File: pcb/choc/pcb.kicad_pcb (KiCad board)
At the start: 2 copper layers, 154.2 x 86 mm, 70 parts, among them J1 MJ-4PP-9, J2 USB_C_Receptacle_USB2.0, J3 Conn_01x04_Female, J4 Conn_01x08_Female, SW1 SW_PUSH, SW10 SW_PUSH, SW11 SW_PUSH, SW12 SW_PUSH, SW13 SW_PUSH, SW14 SW_PUSH, SW15 SW_PUSH, SW16 SW_PUSH, SW17 SW_PUSH, SW18 SW_PUSH, SW19 SW_PUSH, SW2 SW_PUSH, SW3 SW_PUSH, SW4 SW_PUSH, SW5 SW_PUSH, SW6 SW_PUSH, SW7 SW_PUSH, SW8 SW_PUSH, SW9 SW_PUSH, U1 rp2040-zero, U2 rp2040-zero, U3 roller

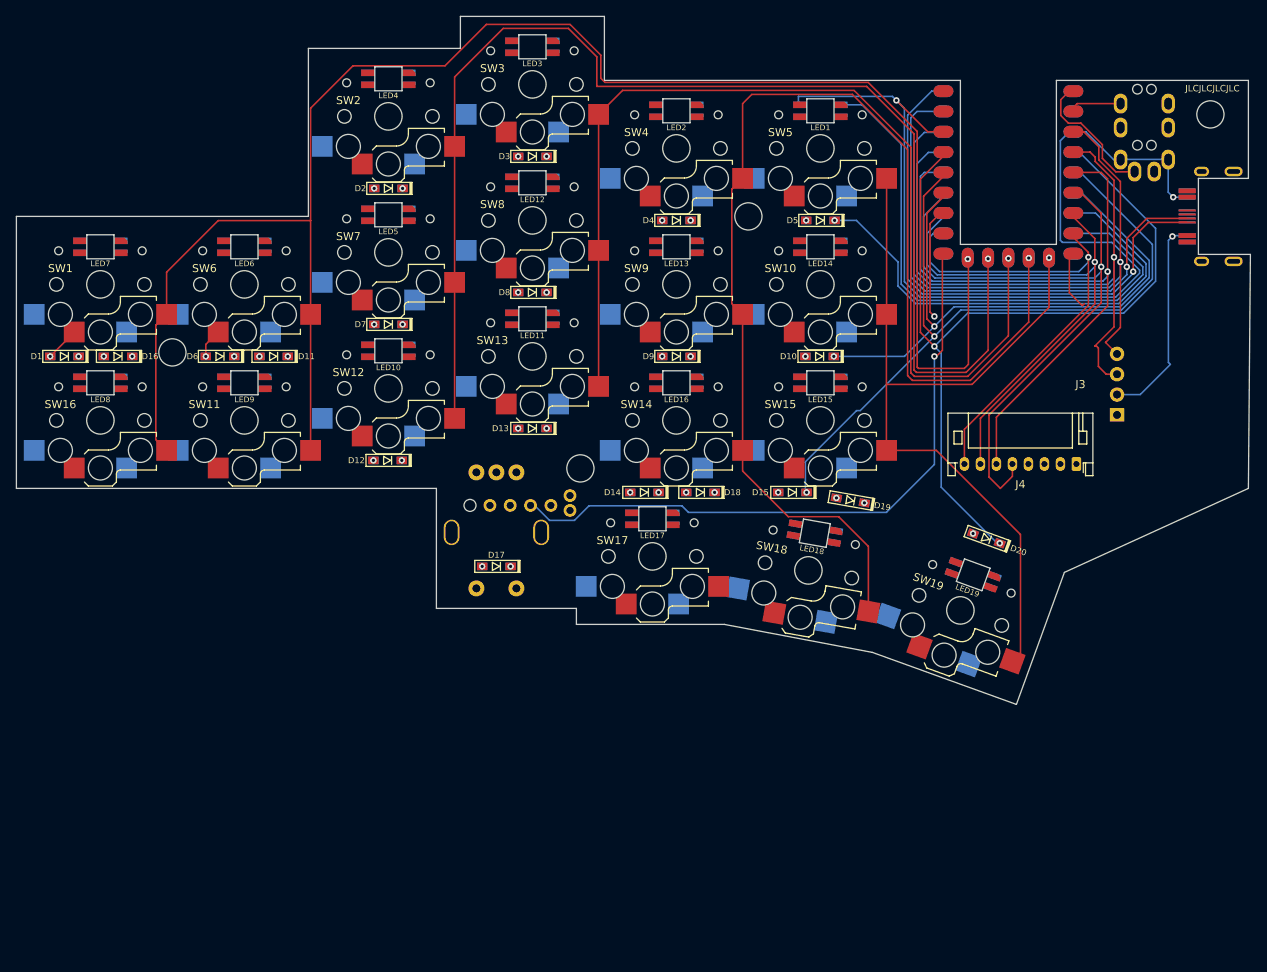
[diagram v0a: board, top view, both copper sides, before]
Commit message: prototype 1
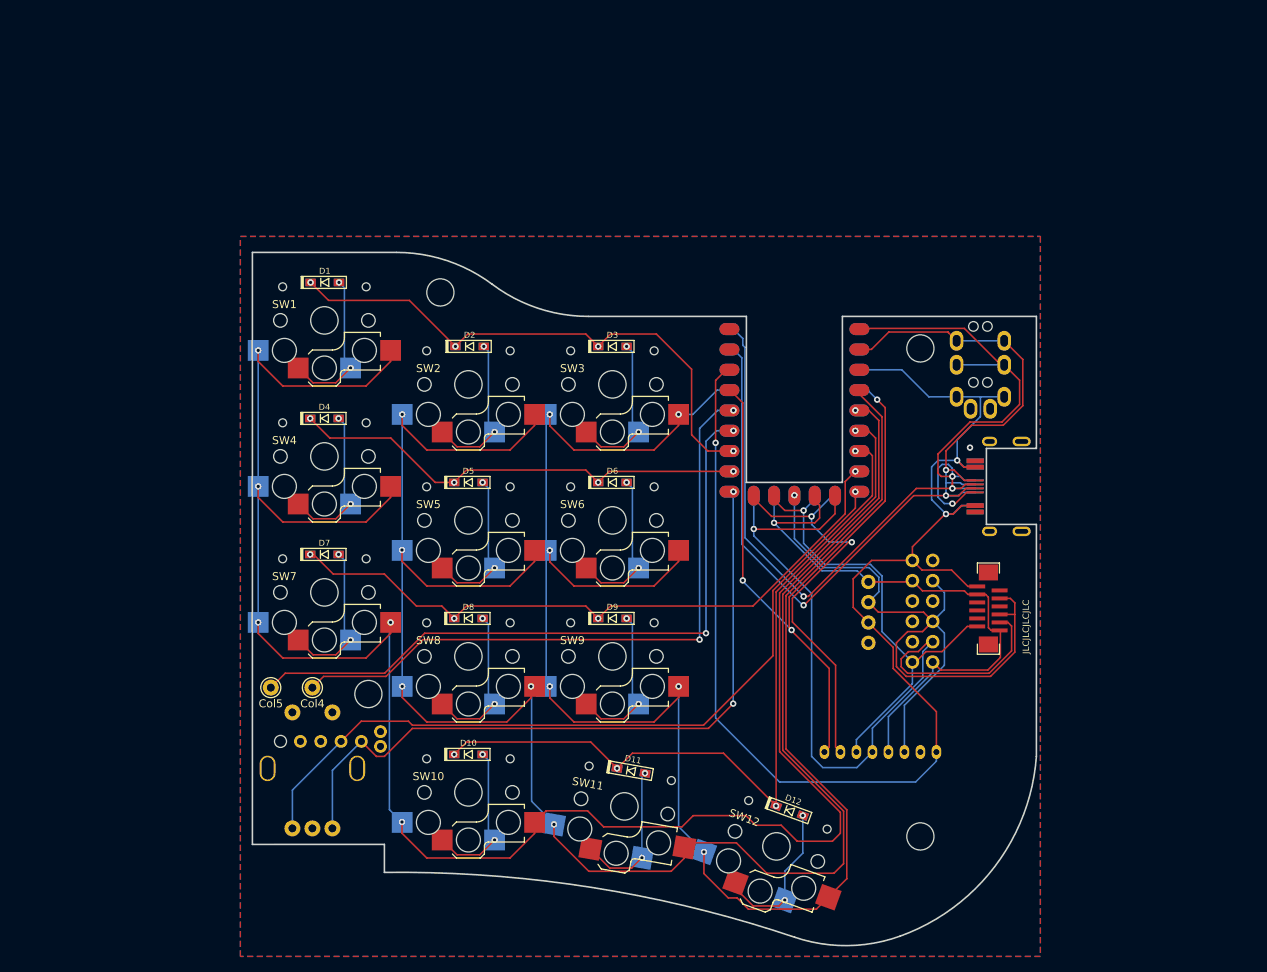
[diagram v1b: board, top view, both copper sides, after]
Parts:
- removed the D1 at (59.0, 82.0)
- removed the D11 at (85.2, 82.0)
- removed the D12 at (99.4, 95.0)
- removed D16, D17: D_Small, zzkeeb:Diode_1N4148-SOD123-reversible
- removed the D2 at (99.5, 61.0)
- removed the D6 at (78.5, 82.0)
- removed the D7 at (99.5, 78.0)
- removed J3: Conn_01x04_Female, zzkeeb:Pointing_Cirque-adapter
- removed J4: Conn_01x08_Female, Connector_JST:JST_PH_S8B-PH-K_1x08_P2.00mm_Horizontal
- removed LED1, LED10, LED11, LED12, LED13, LED14, LED15, LED16, LED17, LED18, LED19, LED2, LED3, LED4, LED5, LED6, LED7, LED8, LED9: YS-SK6812MINI-E, zzkeeb:LED_SK6812-MINI-E-reversible
- removed the SW1 at (63.5, 73.0)
- removed the SW11 at (81.5, 90.0)
- removed the SW12 at (99.5, 86.0)
- removed SW16: SW_PUSH, zzkeeb:Switch_ChocV1-hotswap-reversible
- removed the SW2 at (99.5, 52.0)
- removed the SW6 at (81.5, 73.0)
- removed the SW7 at (99.5, 69.0)
- added CIRQUE1: Conn_01x12_Female, zzkeeb:Connector_FFC-FPC-vertical-12pin, F.Cu at (174.5, 113.5)
- added CIRQUE2: Conn_01x12_Female, zzkeeb:Connector_FPC-FFC-adapter-12pin, F.Cu at (165.0, 107.5)
- added Col4: Conn_01x01_Female, Connector_Pin:Pin_D1.0mm_L10.0mm, F.Cu at (90.0, 123.4)
- added Col5: Conn_01x01_Female, Connector_Pin:Pin_D1.0mm_L10.0mm, F.Cu at (84.8, 123.4)
- added DISP1: Conn_01x08_Female, zzkeeb:Connector_JST_PH_S8B-PH-K_1x08_P2.00mm_Horizontal, F.Cu at (168.0, 131.5)
- added I2C1: Conn_01x04_Female, zzkeeb:Pointing_Cirque-adapter-reversible, F.Cu at (159.5, 110.2)
- D1: renamed from D3; moved to B.Cu
- D10: renamed from D18; moved to B.Cu
- D11: renamed from D19; moved to B.Cu
- D12: renamed from D20; moved to B.Cu
- D2: renamed from D4; moved to B.Cu
- D3: renamed from D5; moved to B.Cu
- D4: renamed from D8; moved to B.Cu
- D5: renamed from D9; moved to B.Cu
- D6: renamed from D10; moved to B.Cu
- D7: renamed from D13; moved to B.Cu
- D8: renamed from D14; moved to B.Cu
- D9: renamed from D15; moved to B.Cu
- MCU1: renamed from U1; moved to F.Cu
- MCU2: renamed from U2; moved to B.Cu
- RE1: footprint zzkeeb:RotaryEncoder_EC11 -> zzkeeb:RotaryEncoder_EC11-reversible
- ROLL1: renamed from U3; footprint zzkeeb:RotaryEncoder_EVQWGD001 -> zzkeeb:RotaryEncoder_EVQWGD001-reversible
- SW1: renamed from SW3; value SW_PUSH -> Switch
- SW10: renamed from SW17; value SW_PUSH -> Switch
- SW11: renamed from SW18; value SW_PUSH -> Switch
- SW12: renamed from SW19; value SW_PUSH -> Switch
- SW2: renamed from SW4; value SW_PUSH -> Switch
- SW3: renamed from SW5; value SW_PUSH -> Switch
- SW4: renamed from SW8; value SW_PUSH -> Switch
- SW5: renamed from SW9; value SW_PUSH -> Switch
- SW6: renamed from SW10; value SW_PUSH -> Switch
- SW7: renamed from SW13; value SW_PUSH -> Switch
- SW8: renamed from SW14; value SW_PUSH -> Switch
- SW9: renamed from SW15; value SW_PUSH -> Switch
- TRRS1: renamed from J1; value MJ-4PP-9 -> AudioJack4
- moved H2 62.6 mm to (166.0, 142.0)
- moved H3 49.2 mm to (97.0, 124.2)
- moved H1 46.6 mm to (166.0, 81.0)
- moved D10 43.7 mm to (109.5, 131.8), turned to 0 degrees
- moved D11 43.5 mm to (129.8, 133.8), turned to -10 degrees
- moved USB1 42.9 mm to (176.0, 98.2)
- moved D12 42.0 mm to (149.6, 138.8), turned to -20 degrees
- moved MCU1 40.0 mm to (150.2, 88.8), turned to 0 degrees
- moved MCU2 40.0 mm to (150.2, 88.8), turned to 180 degrees
- moved H4 39.7 mm to (106.0, 74.0)
- moved SW1 39.3 mm to (91.5, 77.5)
- moved SW2 39.3 mm to (109.5, 85.5)
- moved SW3 39.3 mm to (127.5, 85.5)
- moved SW4 39.3 mm to (91.5, 94.5)
- moved SW5 39.3 mm to (109.5, 102.5)
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- renumbered J2 to USB1
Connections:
- MCU1 pad 10: col0 -> CS
- MCU1 pad 11: col1 -> SCLK/SDA
- MCU1 pad 12: col2 -> MOSI/SCL
- MCU1 pad 13: col3 -> MISO
- MCU1 pad 14: col4 -> RST
- MCU1 pad 16: LED -> row1
- MCU1 pad 18: row1 -> col5
- MCU1 pad 19: row2 -> col4
- MCU1 pad 20: row3 -> BL
- MCU1 pad 3: SCLK/SDA -> unconnected-(MCU1-Pad3)
- MCU1 pad 4: MOSI/SCL -> col2
- MCU1 pad 5: MISO/DC -> col1
- MCU1 pad 6: CS -> col0
- MCU1 pad 7: RST -> row3
- MCU1 pad 8: BL -> row2
- MCU2 pad 10: col4 -> CS
- MCU2 pad 11: col3 -> SCLK/SDA
- MCU2 pad 12: col2 -> MOSI/SCL
- MCU2 pad 13: col1 -> MISO
- MCU2 pad 14: col0 -> RST
- MCU2 pad 16: LED -> row2
- MCU2 pad 17: row0 -> row3
- MCU2 pad 18: row1 -> col0
- MCU2 pad 19: row2 -> col1
- MCU2 pad 20: row3 -> BL
- MCU2 pad 3: SCLK/SDA -> unconnected-(MCU2-Pad3)
- MCU2 pad 4: MOSI/SCL -> col2
- MCU2 pad 5: MISO/DC -> col4
- MCU2 pad 6: CS -> col5
- MCU2 pad 7: RST -> row0
- MCU2 pad 8: BL -> row1
- RE1 pad A: ENCA -> ENCB
- RE1 pad B: ENCB -> ENCA
- RE1 pad S1: col1 -> unconnected-(RE1-PadS1)
- RE1 pad S2: SW_ENCA -> unconnected-(RE1-PadS2)
- ROLL1 pad S1: col1 -> unconnected-(ROLL1-PadS1)
- ROLL1 pad S2: SW_ENCA -> unconnected-(ROLL1-PadS2)
- SW1 pad 2: col2 -> col0
- SW10 pad 2: col2 -> col0
- SW11 pad 2: col3 -> col1
- SW12 pad 2: col4 -> col2
- SW2 pad 2: col3 -> col1
- SW3 pad 2: col4 -> col2
- SW4 pad 2: col2 -> col0
- SW5 pad 2: col3 -> col1
- SW6 pad 2: col4 -> col2
- SW7 pad 2: col2 -> col0
- SW8 pad 2: col3 -> col1
- SW9 pad 2: col4 -> col2
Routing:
- net col3: track 154.0 -> 0.00 mm, vias 1 -> 0
- net col2: track 130.2 -> 223.0 mm, vias 1 -> 6
- net MISO/DC: track 86.6 -> 0.00 mm, vias 1 -> 0
- net col5: track 0.00 -> 85.2 mm, vias 0 -> 2
- net ENCA: track 7.54 -> 88.9 mm, vias 0 -> 2
- net LED: track 71.3 -> 0.00 mm
- net col1: track 162.4 -> 228.4 mm, vias 1 -> 6
- net MISO: track 0.00 -> 60.2 mm, vias 0 -> 1
- net TX: track 85.4 -> 133.6 mm, vias 1 -> 4
- net RX: track 73.3 -> 121.5 mm, vias 1 -> 3
- net VCC: track 148.9 -> 182.2 mm
- net col0: track 224.3 -> 249.6 mm, vias 1 -> 6
- net BL: track 63.1 -> 88.0 mm, vias 1 -> 3
- net col4: track 102.4 -> 82.4 mm, vias 1 -> 2
- net Net-(D12-Pad2): track 0.00 -> 19.6 mm, vias 1 -> 2
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- added copper zone on B.Cu, net GND
- added copper zone on F.Cu, net GND
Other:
- board size 154.2 x 86 mm -> 98 x 86.7 mm
